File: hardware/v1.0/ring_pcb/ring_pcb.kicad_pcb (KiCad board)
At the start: 2 copper layers, 17.8 x 17.8 mm, 18 parts

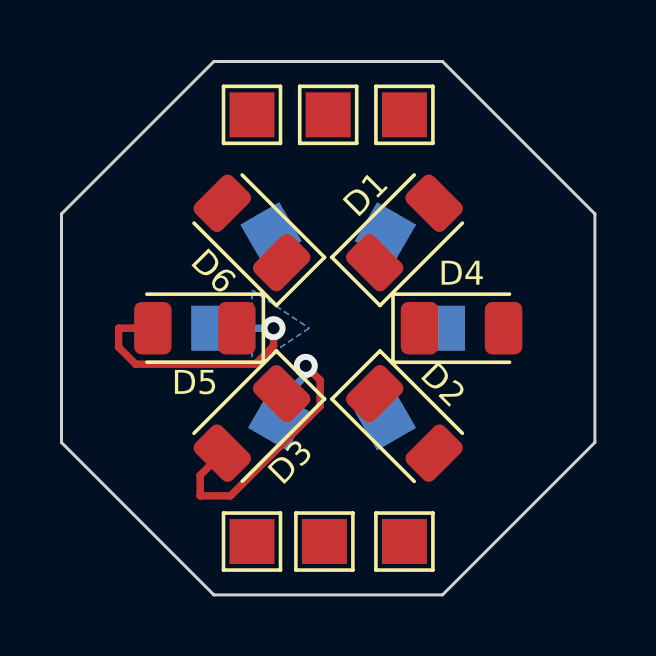
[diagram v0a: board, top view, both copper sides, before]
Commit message: New PCB and Gerbers
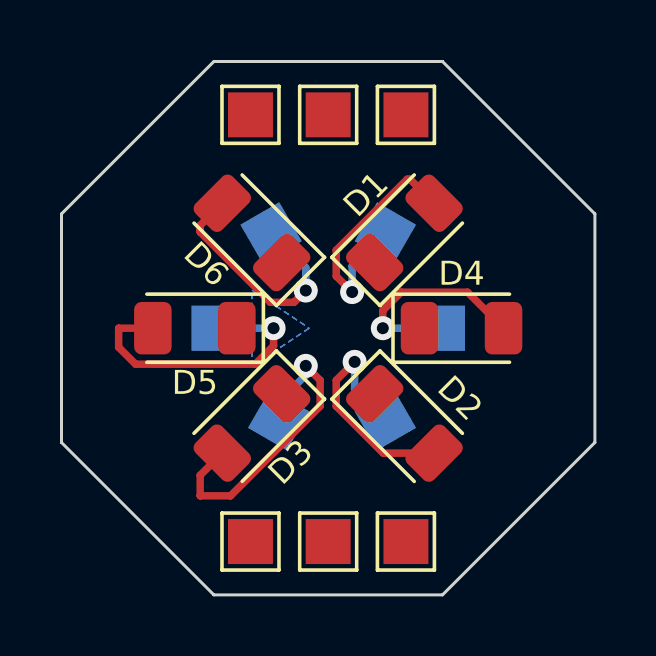
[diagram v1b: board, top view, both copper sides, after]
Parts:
- moved TP8 0.13 mm to (137.2, 106.2)
- moved TP10 0.05 mm to (139.8, 91.9)
- moved TP11 0.05 mm to (134.6, 106.2)
- moved TP12 0.05 mm to (134.6, 91.9)
- moved TP9 0.05 mm to (139.8, 106.2)
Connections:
- net Net-(D1-Pad2) renamed /N1
- net Net-(D3-Pad2) renamed /N3
- net Net-(D4-Pad2) renamed /N4
- net Net-(D5-Pad2) renamed /N5
- net Net-(D6-Pad2) renamed /N6
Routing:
- net /N1: track 0.00 -> 8.62 mm, vias 0 -> 1
- net /N6: track 0.00 -> 8.32 mm, vias 0 -> 1
- net /N2: track 0.00 -> 7.99 mm, vias 0 -> 1
- net /N4: track 0.00 -> 7.35 mm, vias 0 -> 1
